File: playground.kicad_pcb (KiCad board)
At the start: 2 copper layers, 50 x 50 mm, 20 parts, among them IC1 TXU0101DBVR, IC3 TXU0101DBVR, IC4 TXU0101DBVR, IC5 TXU0101DBVR, IC6 TXU0101DBVR, IC7 TXU0101DBVR, IC8 TXU0101DBVR, J1 USB_A, SW1 SW_DIP_x01, U2 ATSAMD21G18A-A

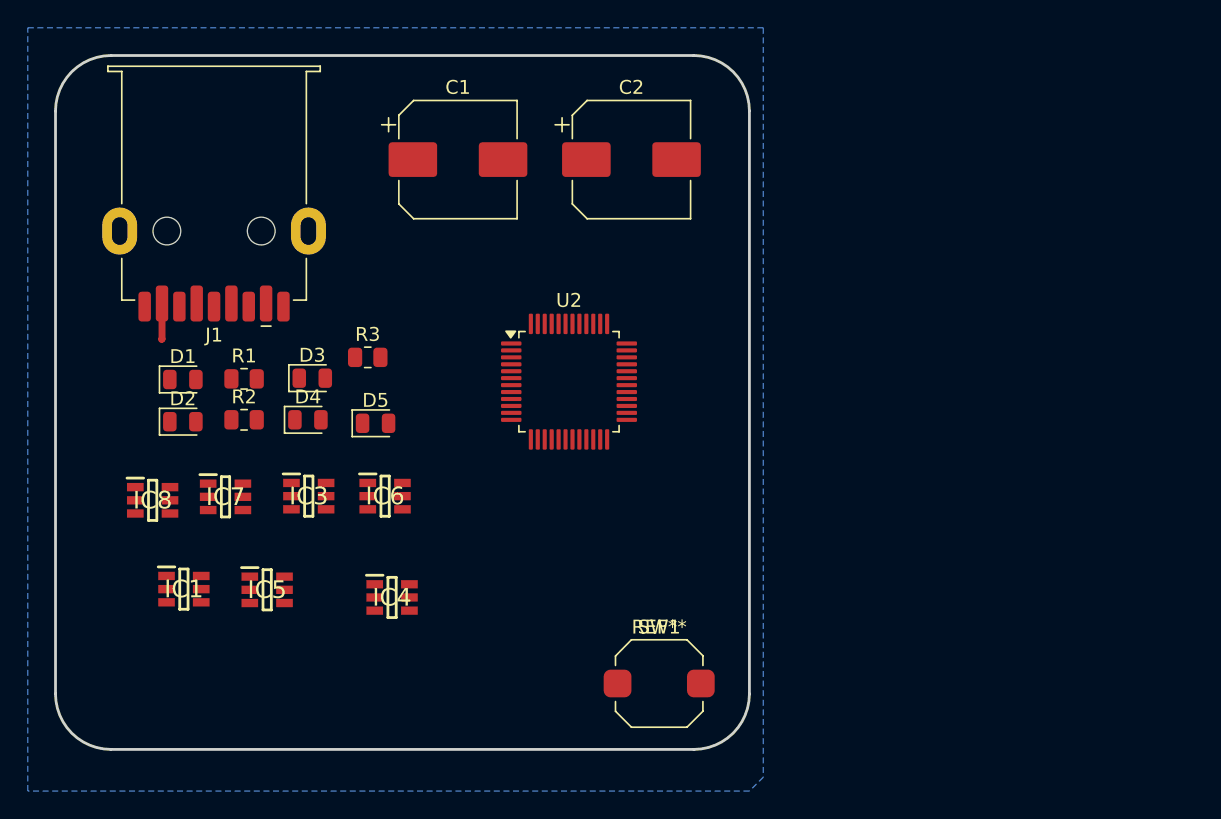
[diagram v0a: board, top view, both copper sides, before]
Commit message: updates
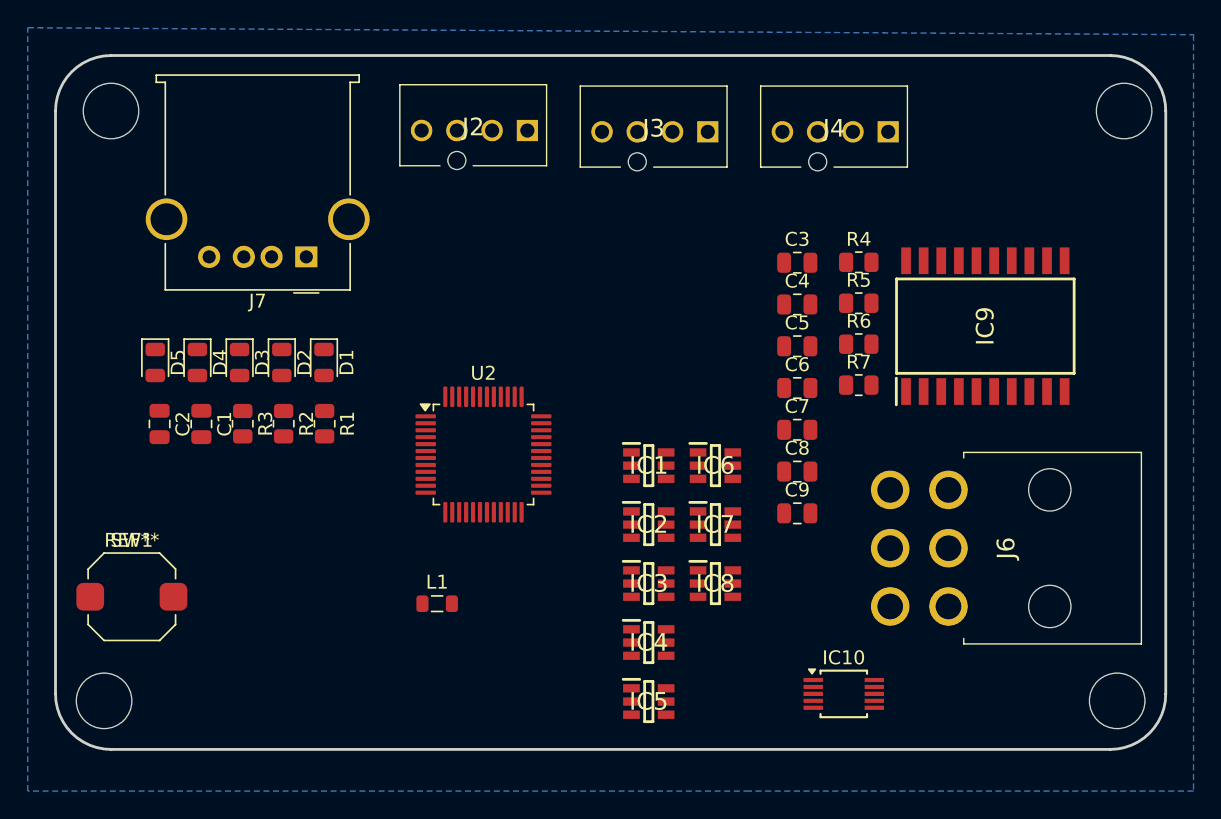
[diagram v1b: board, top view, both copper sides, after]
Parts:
- removed J1: USB_A, Connector_USB:USB3_A_Receptacle_Wuerth_692122030100
- added C3: 10u, Capacitor_SMD:C_0805_2012Metric, F.Cu at (153.4, 64.9)
- added C4: 10u, Capacitor_SMD:C_0805_2012Metric, F.Cu at (153.4, 67.9)
- added C5: 100n, Capacitor_SMD:C_0805_2012Metric, F.Cu at (153.4, 71.0)
- added C6: 100n, Capacitor_SMD:C_0805_2012Metric, F.Cu at (153.4, 74.0)
- added C7: 33p, Capacitor_SMD:C_0805_2012Metric, F.Cu at (153.4, 77.0)
- added C8: 22u, Capacitor_SMD:C_0805_2012Metric, F.Cu at (153.4, 80.0)
- added C9: 100n, Capacitor_SMD:C_0805_2012Metric, F.Cu at (153.4, 83.0)
- added IC10: TPS562242DRLR, Package_SO:MSOP-10_3x3mm_P0.5mm, F.Cu at (156.8, 96.0)
- added IC2: TXU0101DBVR, custom_footprints:TXU0101DBVR, F.Cu at (142.8, 83.8)
- added IC9: L293DD, custom_footprints:SOIC127P1032X265-20N, F.Cu at (167.0, 69.5)
- added J2: Pump, custom_footprints:470531000, F.Cu at (134.0, 55.4)
- added J3: Fan, custom_footprints:470531000, F.Cu at (147.0, 55.5)
- added J4: Valve, custom_footprints:470531000, F.Cu at (160.0, 55.5)
- added J6: MOLEX POWER CONNECTOR, custom_footprints:455580003, F.Cu at (164.3, 81.3)
- added J7: USB_A, Connector_USB:USB_A_Molex_67643_Horizontal, F.Cu at (118.1, 64.5)
- added L1: 3u3, Inductor_SMD:L_0805_2012Metric, F.Cu at (127.5, 89.5)
- added R4: 100k, Resistor_SMD:R_0805_2012Metric, F.Cu at (157.9, 64.9)
- added R5: 11k3, Resistor_SMD:R_0805_2012Metric, F.Cu at (157.9, 67.8)
- added R6: 158k, Resistor_SMD:R_0805_2012Metric, F.Cu at (157.9, 70.8)
- added R7: 30k, Resistor_SMD:R_0805_2012Metric, F.Cu at (157.9, 73.8)
- C1, C2: footprint Capacitor_SMD:CP_Elec_8x10 -> Capacitor_SMD:C_0805_2012Metric
- moved IC8 41.0 mm to (147.6, 88.0)
- moved C2 39.0 mm to (107.5, 76.5), turned to -90 degrees
- moved SW1 38.5 mm to (105.5, 89.0)
- moved IC7 35.4 mm to (147.6, 83.8)
- moved IC1 34.7 mm to (142.8, 79.5)
- moved IC5 28.7 mm to (142.8, 96.5)
- moved C1 26.5 mm to (110.5, 76.5), turned to -90 degrees
- moved IC3 25.3 mm to (142.8, 88.0)
- moved IC6 23.9 mm to (147.6, 79.5)
- moved IC4 18.8 mm to (142.8, 92.3)
- moved D5 16.5 mm to (107.2, 72.1), turned to -90 degrees
- moved D1 10.2 mm to (119.3, 72.1), turned to -90 degrees
- moved R3 10.2 mm to (113.5, 76.5), turned to -90 degrees
- moved D4 8.97 mm to (110.2, 72.1), turned to -90 degrees
- moved D2 8.31 mm to (116.3, 72.1), turned to -90 degrees
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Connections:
- IC1 pad 1: +3V3 -> +5V
- IC1 pad 3: /PumpCtrl_3v3 -> /PumpSense_5v
- IC1 pad 4: /PumpCtrl_5v -> /PumpSense_3v3
- IC1 pad 5: +5V -> +3V3
- IC1 pad 6: +5V -> +3V3
- IC3 pad 1: +3V3 -> +5V
- IC3 pad 3: /ValveCtrl1_3v3 -> /ValveSense1_5v
- IC3 pad 4: /ValveCtrl1_5v -> /ValveSense1_3v3
- IC3 pad 5: +5V -> +3V3
- IC3 pad 6: +5V -> +3V3
- IC4 pad 1: +3V3 -> +5V
- IC4 pad 3: /ValveCtrl2_3v3 -> /ValveSense2_5v
- IC4 pad 4: /ValveCtrl2_5v -> /ValveSense2_3v3
- IC4 pad 5: +5V -> +3V3
- IC4 pad 6: +5V -> +3V3
- IC5 pad 1: +5V -> +3V3
- IC5 pad 3: /PumpSense_5v -> /PumpCtrl_3v3
- IC5 pad 4: /PumpSense_3v3 -> /PumpCtrl_5v
- IC5 pad 5: +3V3 -> +5V
- IC5 pad 6: +3V3 -> +5V
- IC6 pad 1: +5V -> +3V3
- IC6 pad 3: /FanSense_5v -> /FanCtrl_3v3
- IC6 pad 4: /FanSense_3v3 -> /FanCtrl_5v
- IC6 pad 5: +3V3 -> +5V
- IC6 pad 6: +3V3 -> +5V
- IC7 pad 1: +5V -> +3V3
- IC7 pad 3: /ValveSense1_5v -> /ValveCtrl1_3v3
- IC7 pad 4: /ValveSense1_3v3 -> /ValveCtrl1_5v
- IC7 pad 5: +3V3 -> +5V
- IC7 pad 6: +3V3 -> +5V
- IC8 pad 1: +5V -> +3V3
- IC8 pad 3: /ValveSense2_5v -> /ValveCtrl2_3v3
- IC8 pad 4: /ValveSense2_3v3 -> /ValveCtrl2_5v
- IC8 pad 5: +3V3 -> +5V
- IC8 pad 6: +3V3 -> +5V
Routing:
- net GND: track 2.60 -> 0.00 mm
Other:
- board size 50 x 50 mm -> 80 x 50 mm
